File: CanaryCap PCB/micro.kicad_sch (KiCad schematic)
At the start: 22 parts, among them SW1 SW_MEC_5E, SW2 SW_MEC_5E, U3 ESP32-C6FH4

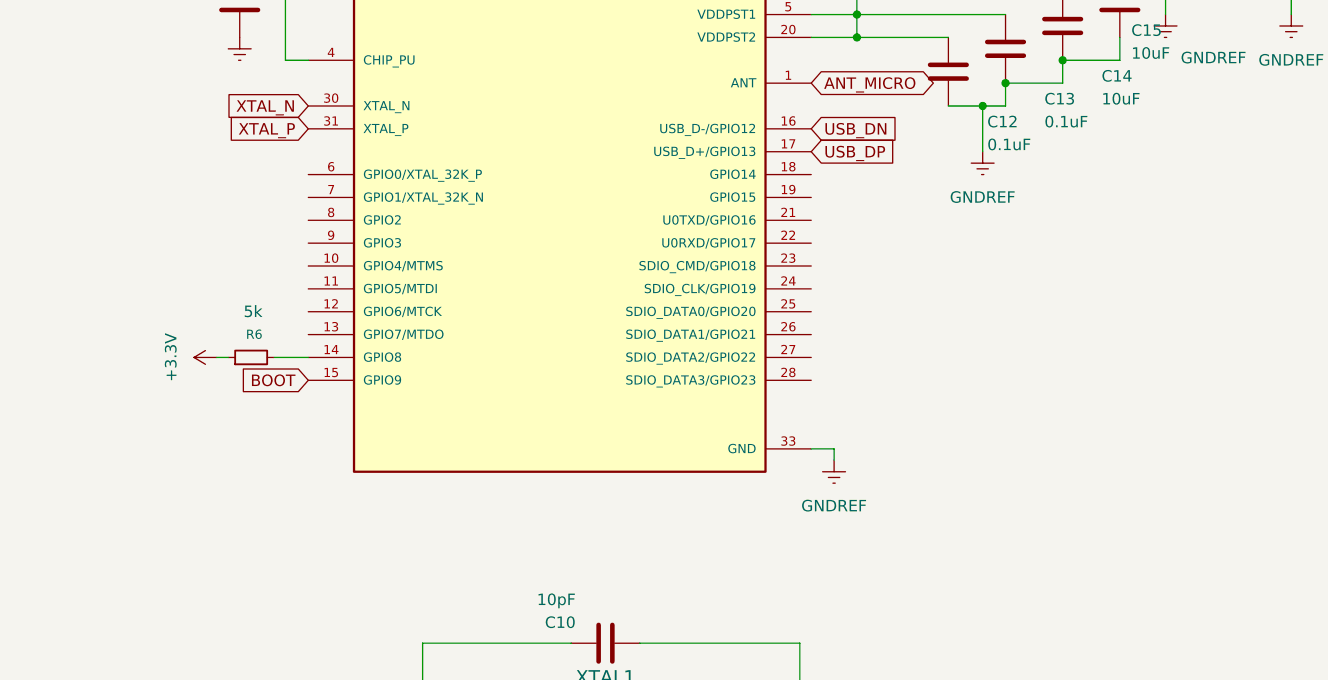
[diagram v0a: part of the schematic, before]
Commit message: new changes
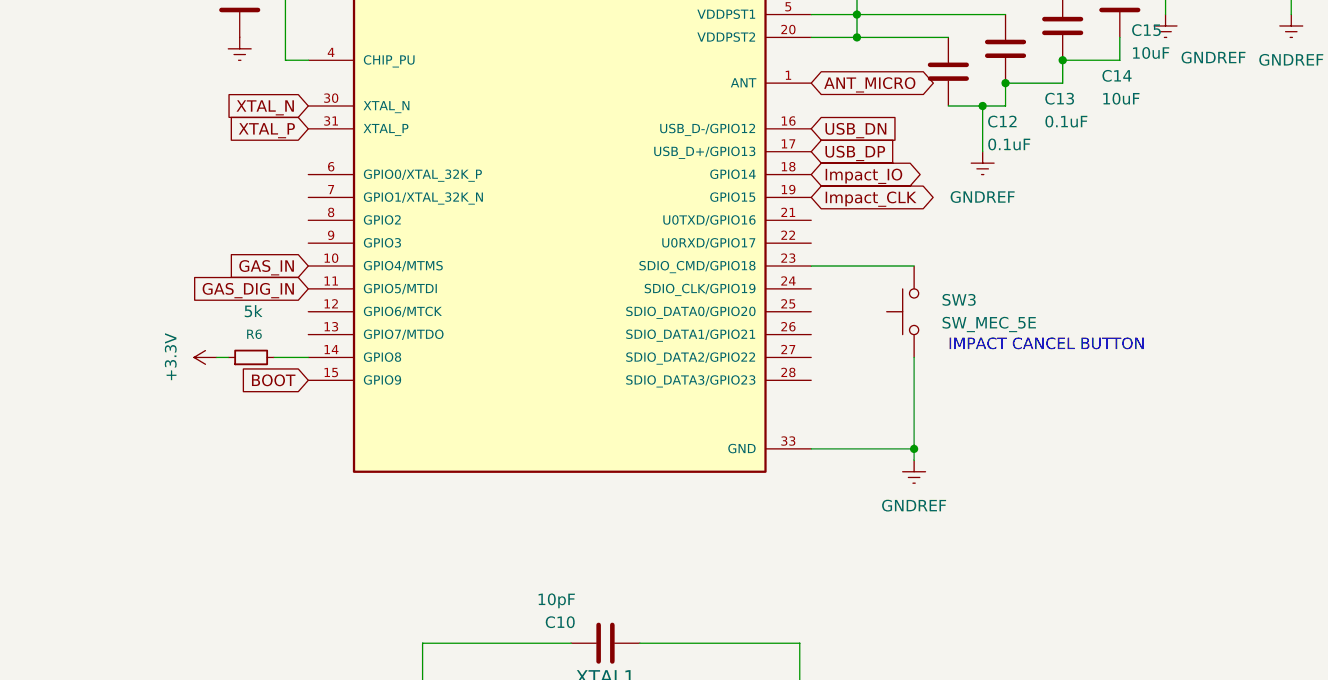
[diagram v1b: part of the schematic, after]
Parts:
- added SW3: SW_MEC_5E, Button_Switch_SMD:SW_SPST_EVQP2_MiddlePushTravel_H2.5mm, symbol Switch:SW_Push
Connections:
- net GNDREF: now also SW3.1
- net GAS_IN: now reaches U3.10 (GPIO4/MTMS)
- net GAS_DIG_IN: now reaches U3.11 (GPIO5/MTDI)
- net Impact_IO: now reaches U3.18 (GPIO14)
- net Impact_CLK: now reaches U3.19 (GPIO15)
- net at U3.23 (SDIO_CMD/GPIO18): now also SW3.2
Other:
- note added: "IMPACT CANCEL BUTTON"
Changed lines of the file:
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@@
 		(comment 1 "Sebastian Arthur")
+	)
+	(text "IMPACT CANCEL BUTTON\n"
+		(exclude_from_sim no)
+		(at 223.012 87.63 0)
+		(effects
+			(font
+				(size 1.27 1.27)
+			)
+		)
 	)
 	(text "NP0/C0G Capacitor for high speed and accuracy"
@@
 	)
 	(junction
+		(at 208.28 99.06)
+		(diameter 0)
+		(color 0 0 0 0)
+	)
+	(junction
 		(at 236.22 40.64)
 		(diameter 0)
@@
 	(wire
 		(pts
+			(xy 208.28 88.9) (xy 208.28 99.06)
+		)
+		(stroke
+			(width 0)
+			(type default)
+		)
+	)
+	(wire
+		(pts
 			(xy 151.13 134.62) (xy 153.67 134.62)
 		)
@@
 	(wire
 		(pts
+			(xy 196.85 78.74) (xy 208.28 78.74)
+		)
+		(stroke
+			(width 0)
+			(type default)
+		)
+	)
+	(wire
+		(pts
 			(xy 153.67 137.16) (xy 153.67 151.13)
 		)
@@
 	(wire
 		(pts
-			(xy 196.85 99.06) (xy 199.39 99.06)
+			(xy 196.85 99.06) (xy 208.28 99.06)
 		)
 		(stroke
@@
 	(wire
 		(pts
-			(xy 199.39 99.06) (xy 199.39 100.33)
+			(xy 208.28 99.06) (xy 208.28 100.33)
 		)
 		(stroke
@@
 		)
 	)
+	(global_label "Impact_CLK"
+		(shape bidirectional)
+		(at 196.85 71.12 0)
+		(fields_autoplaced yes)
+		(effects
+			(font
+				(size 1.27 1.27)
+			)
+			(justify left)
+		)
+		(property "Intersheetrefs" "${INTERSHEET_REFS}"
+			(at 211.8926 71.12 0)
+			(effects
+				(font
+					(size 1.27 1.27)
+				)
+				(justify left)
+				(hide yes)
+			)
+		)
+	)
+	(global_label "GAS_IN"
+		(shape input)
+		(at 140.97 78.74 180)
+		(fields_autoplaced yes)
+		(effects
+			(font
+				(size 1.27 1.27)
+			)
+			(justify right)
+		)
+		(property "Intersheetrefs" "${INTERSHEET_REFS}"
+			(at 131.5138 78.74 0)
+			(effects
+				(font
+					(size 1.27 1.27)
+				)
+				(justify right)
+				(hide yes)
+			)
+		)
+	)
+	(global_label "GAS_DIG_IN"
+		(shape input)
+		(at 140.97 81.28 180)
+		(fields_autoplaced yes)
+		(effects
+			(font
+				(size 1.27 1.27)
+			)
+			(justify right)
+		)
+		(property "Intersheetrefs" "${INTERSHEET_REFS}"
+			(at 127.4014 81.28 0)
+			(effects
+				(font
+					(size 1.27 1.27)
+				)
+				(justify right)
+				(hide yes)
+			)
+		)
+	)
 	(global_label "BOOT"
 		(shape output)
@@
 				)
 				(justify right)
+				(hide yes)
+			)
+		)
+	)
+	(global_label "Impact_IO"
+		(shape bidirectional)
+		(at 196.85 68.58 0)
+		(fields_autoplaced yes)
+		(effects
+			(font
+				(size 1.27 1.27)
+			)
+			(justify left)
+		)
+		(property "Intersheetrefs" "${INTERSHEET_REFS}"
+			(at 210.2598 68.58 0)
+			(effects
+				(font
+					(size 1.27 1.27)
+				)
+				(justify left)
 				(hide yes)
 			)
@@
 	)
 	(symbol
+		(lib_id "Switch:SW_Push")
+		(at 208.28 83.82 90)
+		(unit 1)
+		(exclude_from_sim no)
+		(in_bom yes)
+		(on_board yes)
+		(dnp no)
+		(property "Reference" "SW3"
+			(at 211.328 82.55 90)
+			(effects
+				(font
+					(size 1.27 1.27)
+				)
+				(justify right)
+			)
+		)
+		(property "Value" "SW_MEC_5E"
+			(at 211.328 85.09 90)
+			(effects
+				(font
+					(size 1.27 1.27)
+				)
+				(justify right)
+			)
+		)
+		(property "Footprint" "Button_Switch_SMD:SW_SPST_EVQP2_MiddlePushTravel_H2.5mm"
+			(at 203.2 83.82 0)
+			(effects
+				(font
+					(size 1.27 1.27)
+				)
+				(hide yes)
+			)
+		)
+		(property "Datasheet" "~"
+			(at 203.2 83.82 0)
+			(effects
+				(font
+					(size 1.27 1.27)
+				)
+				(hide yes)
+			)
+		)
+		(property "Description" "Push button switch, generic, two pins"
+			(at 208.28 83.82 0)
+			(effects
+				(font
+					(size 1.27 1.27)
+				)
+				(hide yes)
+			)
+		)
+		(pin "1"
+		)
+		(pin "2"
+		)
+		(instances
+			(project "CanaryCap"
+				(path "/406ad30e-b04c-4bb7-9588-aab8ab73084a/865b4f90-0093-4030-8a8d-928bbea99e0f"
+					(reference "SW3")
+					(unit 1)
+				)
+			)
+		)
+	)
+	(symbol
 		(lib_id "Device:R_Small")
 		(at 134.62 88.9 90)
@@
 	(symbol
 		(lib_id "power:GNDREF")
-		(at 199.39 100.33 0)
+		(at 208.28 100.33 0)
 		(unit 1)
 		(exclude_from_sim no)
@@
 		(fields_autoplaced yes)
 		(property "Reference" "#PWR018"
-			(at 199.39 106.68 0)
+			(at 208.28 106.68 0)
 			(effects
 				(font
@@
 		)
 		(property "Value" "GNDREF"
-			(at 199.39 105.41 0)
+			(at 208.28 105.41 0)
 			(effects
 				(font
@@
 		)
 		(property "Footprint" ""
-			(at 199.39 100.33 0)
+			(at 208.28 100.33 0)
 			(effects
 				(font
@@
 		)
 		(property "Datasheet" ""
-			(at 199.39 100.33 0)
+			(at 208.28 100.33 0)
 			(effects
 				(font
@@
 		)
 		(property "Description" "Power symbol creates a global label with name \"GNDREF\" , reference supply ground"
-			(at 199.39 100.33 0)
-			(effects
-				(font
+			(at 208.28 100.33 0)
+			(effects
+				(font
